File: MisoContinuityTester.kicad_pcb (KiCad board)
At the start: 2 copper layers, 43.2 x 17.8 mm, 6 parts, among them J1 Analog, J2 Digital

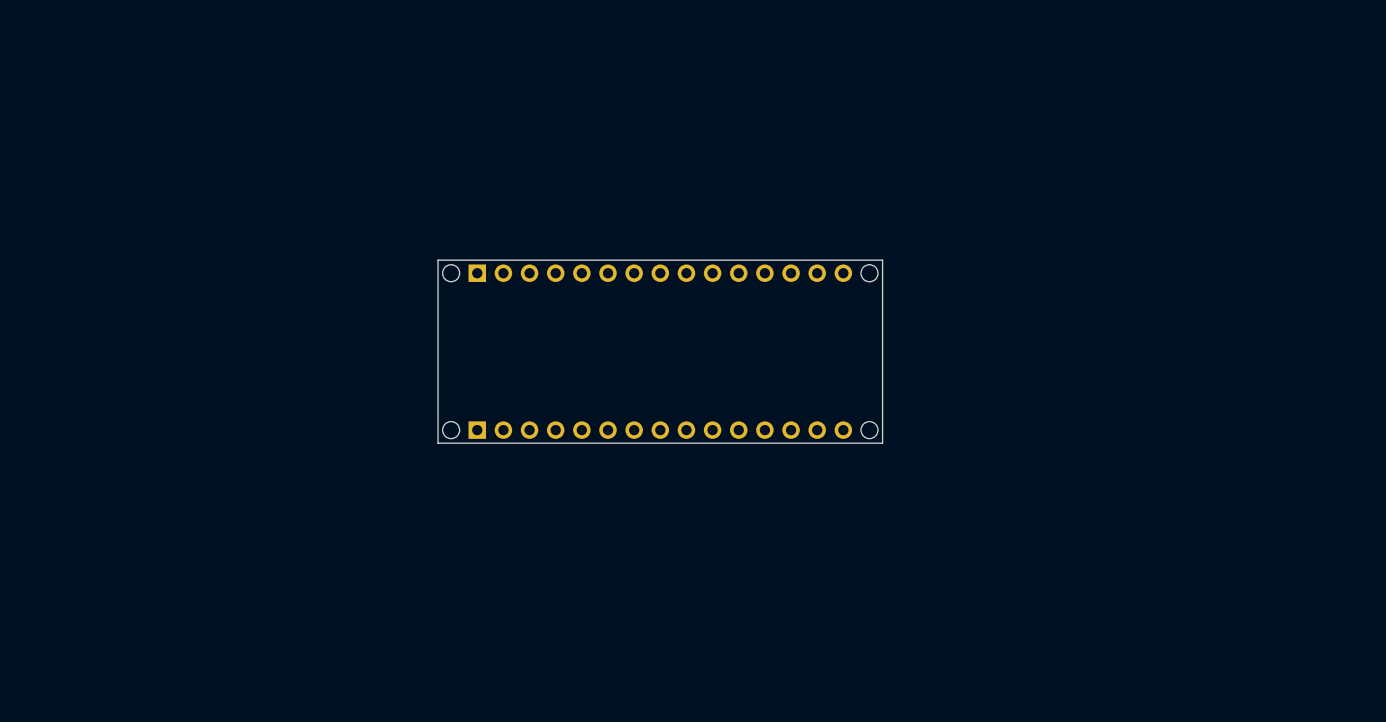
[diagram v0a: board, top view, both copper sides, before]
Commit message: added 3d models, worked on pcb
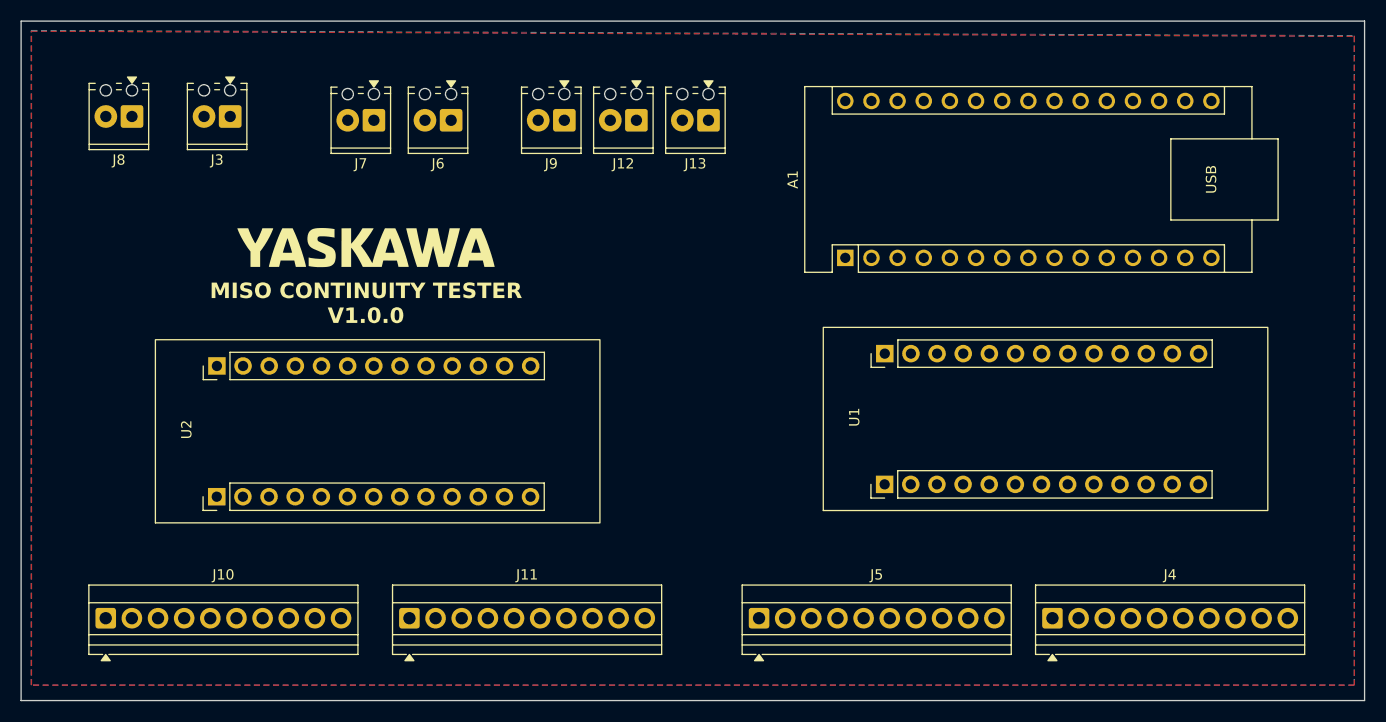
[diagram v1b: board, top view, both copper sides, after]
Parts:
- removed J1: Analog, Connector_PinHeader_2.54mm:PinHeader_1x15_P2.54mm_Vertical
- removed J2: Digital, Connector_PinHeader_2.54mm:PinHeader_1x15_P2.54mm_Vertical
- removed MH1, MH2, MH3, MH4: MountingHole_65mil, Arduino_MountingHole:MountingHole_65mil
- added A1: Arduino_Nano_Every, Module:Arduino_Nano, F.Cu at (139.6, 82.0)
- added G***: LOGO, LOGO, F.Cu at (93.0, 81.0)
- added J10: OUTPUT, TerminalBlock:TerminalBlock_Xinya_XY308-2.54-10P_1x10_P2.54mm_Horizontal, F.Cu at (67.7, 117.0)
- added J11: OUTPUT, TerminalBlock:TerminalBlock_Xinya_XY308-2.54-10P_1x10_P2.54mm_Horizontal, F.Cu at (97.2, 117.0)
- added J12: TYPE1, TerminalBlock_Phoenix:TerminalBlock_Phoenix_MPT-0,5-2-2.54_1x02_P2.54mm_Horizontal, F.Cu at (119.3, 68.6)
- added J13: TYPE2, TerminalBlock_Phoenix:TerminalBlock_Phoenix_MPT-0,5-2-2.54_1x02_P2.54mm_Horizontal, F.Cu at (126.3, 68.6)
- added J3: POWER SWITCH, TerminalBlock_Phoenix:TerminalBlock_Phoenix_MPT-0,5-2-2.54_1x02_P2.54mm_Horizontal, F.Cu at (79.8, 68.3)
- added J4: INPUT, TerminalBlock:TerminalBlock_Xinya_XY308-2.54-10P_1x10_P2.54mm_Horizontal, F.Cu at (159.7, 117.0)
- added J5: INPUT, TerminalBlock:TerminalBlock_Xinya_XY308-2.54-10P_1x10_P2.54mm_Horizontal, F.Cu at (131.2, 117.0)
- added J6: FAIL, TerminalBlock_Phoenix:TerminalBlock_Phoenix_MPT-0,5-2-2.54_1x02_P2.54mm_Horizontal, F.Cu at (101.3, 68.6)
- added J7: PASS, TerminalBlock_Phoenix:TerminalBlock_Phoenix_MPT-0,5-2-2.54_1x02_P2.54mm_Horizontal, F.Cu at (93.8, 68.6)
- added J8: POWER 5V-12V, TerminalBlock_Phoenix:TerminalBlock_Phoenix_MPT-0,5-2-2.54_1x02_P2.54mm_Horizontal, F.Cu at (70.3, 68.3)
- added J9: START, TerminalBlock_Phoenix:TerminalBlock_Phoenix_MPT-0,5-2-2.54_1x02_P2.54mm_Horizontal, F.Cu at (112.3, 68.6)
- added U1: ~, addedItems:Adafruit MCP23017, F.Cu at (143.4, 104.0)
- added U2: ~, addedItems:Adafruit MCP23017, F.Cu at (78.5, 105.2)
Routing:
- added copper zone on B.Cu, net GND
- added copper zone on F.Cu, net VCC
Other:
- board size 43.2 x 17.8 mm -> 130.5 x 66 mm
- board text added: "MISO CONTINUITY TESTER V1.0.0"
- board text removed: "ICSP"
- board text removed: "USB Mini-B"
